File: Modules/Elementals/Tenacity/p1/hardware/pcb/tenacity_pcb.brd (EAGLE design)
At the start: 17.8 x 103.2 mm, 27 parts, among them J1 EURO_POWER, J2 WQP-PJ398SM6, J3 WQP-PJ398SM6, J4 WQP-PJ398SM6, J5 WQP-PJ398SM6, J6 WQP-PJ398SM6, J7 WQP-PJ398SM6, J8 WQP-PJ398SM6, J9 WQP-PJ398SM6, U1 TL072P, U2 TL072P

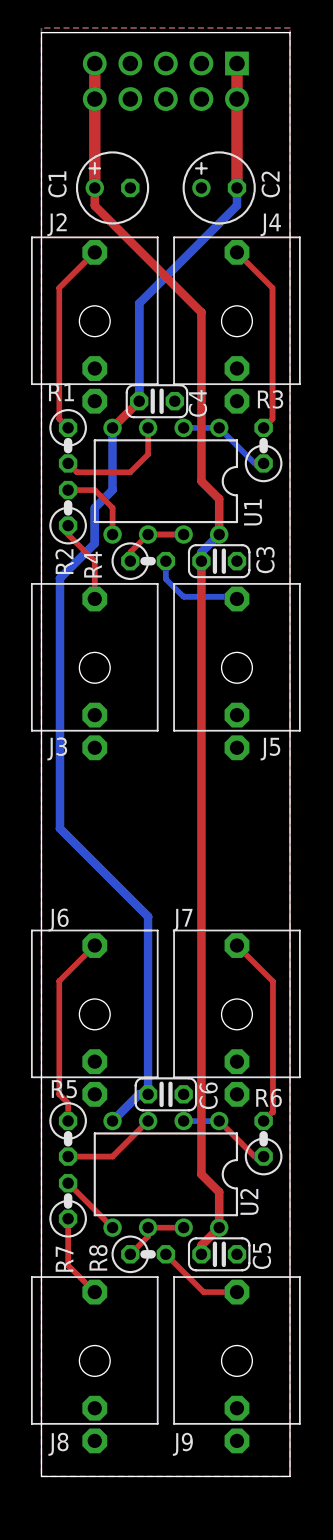
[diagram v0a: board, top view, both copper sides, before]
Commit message: Finalized tenacity p1
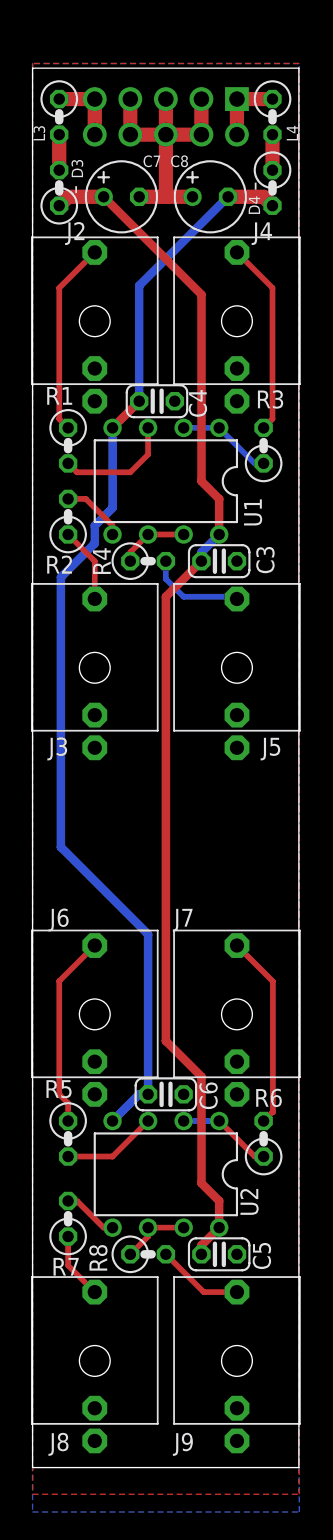
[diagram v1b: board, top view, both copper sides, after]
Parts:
- removed C1, C2: 10u, SonicAthame:TT2D5
- removed J1: EURO_POWER, SonicAthame:EURO_POWER
- added C7, C8: 10u, SonicAthame:TT2D5
- added D3, D4: SB230TA, SonicAthame:0207/2V-POL
- added J10: EURO_POWER, SonicAthame:EURO_POWER
- added L3, L4: 2743005112, SonicAthame:0207/2V
- moved R7 1.27 mm to (3.17, 29.2)
- moved R2 0.64 mm to (3.17, 79.4)
- moved U$2 0.63 mm to (10.2, 59.1)
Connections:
- new net N$21: D3.A, L3.2
- new net N$22: D4.C, L4.2
- new net N$23: J10.1, J10.10, L4.1
- new net N$24: J10.5, J10.6, L3.1
- net +12V: now also C7.+, D3.C; no longer C1.+, J1.5, J1.6
- net -12V: now also C8.-, D4.A; no longer C2.-, J1.1, J1.10
- net GND: now also C7.-, C8.+, J10.2, J10.3, J10.4, J10.7, J10.8, J10.9; no longer C1.-, C2.+, J1.2, J1.3, J1.4, J1.7, J1.8, J1.9
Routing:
- net GND: track 0.00 -> 21.0 mm
- net -12V: track 84.8 -> 78.4 mm
- net N$23: track 0.00 -> 5.08 mm
- net N$24: track 0.00 -> 5.08 mm
- net +12V: track 90.4 -> 86.1 mm
- net N$22: track 0.00 -> 2.54 mm
- net N$21: track 0.00 -> 2.54 mm
- net N$1: track 6.03 -> 4.76 mm
- net N$7: track 5.61 -> 4.60 mm
- net N$11: track 6.03 -> 5.39 mm
- net N$2: track 4.49 -> 3.96 mm
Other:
- board size 17.8 x 103.2 mm -> 19 x 100 mm
- board text added: "STRIPE"
- board text added: "Sonic Athame is fully open-hardware and open-software! Find schematics, code, PCBs, and build instructions at sonic-athame.com"
- board text removed: "Sonic Athame is fully open-hardware and open-software! Find schematics and code on the official GitHub: github.com/nimaid/Sonic-Athame-eurorack"
